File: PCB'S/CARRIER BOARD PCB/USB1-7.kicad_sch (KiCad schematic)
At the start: 7 parts, among them J10 USB_A - 4, J11 USB_A - 5, J12 USB_A - 6 (For Display), J13 USB_A - 7 (For RTL SDR), J14 USB_A - 2 (Extra/For phone ), J7 USB_A - 1, J9 USB_A - 3

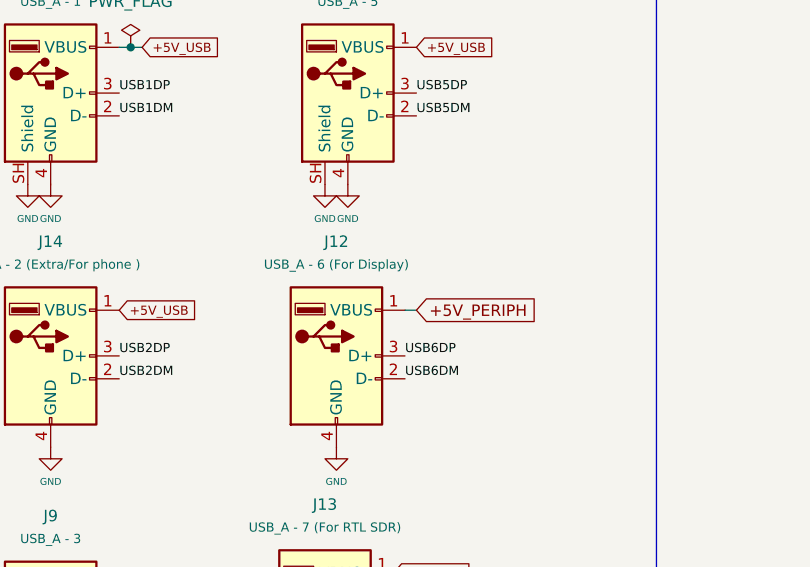
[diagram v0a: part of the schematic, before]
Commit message: ain
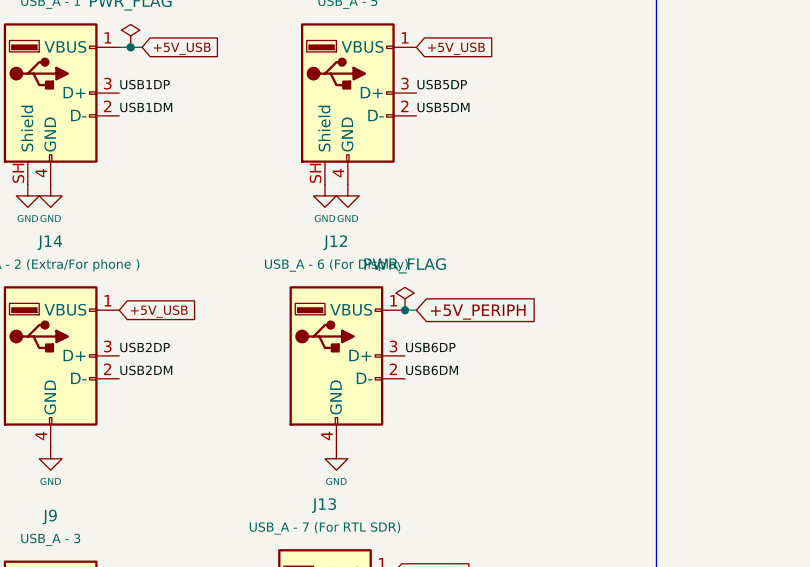
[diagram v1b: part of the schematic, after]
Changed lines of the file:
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@@
+		(color 0 0 0 0)
+	)
+	(junction
+		(at 78.74 92.71)
+		(diameter 0)
 		(color 0 0 0 0)
 	)
@@
 					(unit 1)
 				)
+			)
+		)
+	)
+	(symbol
+		(lib_id "power:PWR_FLAG")
+		(at 78.74 92.71 0)
+		(unit 1)
+		(body_style 1)
+		(exclude_from_sim no)
+		(in_bom yes)
+		(on_board yes)
+		(in_pos_files yes)
+		(dnp no)
+		(fields_autoplaced yes)
+		(property "Reference" "#FLG04"
+			(at 78.74 90.805 0)
+			(hide yes)
+			(show_name no)
+			(do_not_autoplace no)
+			(effects
+				(font
+					(size 1.27 1.27)
+				)
+			)
+		)
+		(property "Value" "PWR_FLAG"
+			(at 78.74 87.63 0)
+			(show_name no)
+			(do_not_autoplace no)
+			(effects
+				(font
+					(size 1.27 1.27)
+				)
+			)
+		)
+		(property "Footprint" "Package_SO:TSSOP-28_4.4x9.7mm_P0.65mm"
+			(at 78.74 92.71 0)
+			(hide yes)
+			(show_name no)
+			(do_not_autoplace no)
+			(effects
+				(font
+					(size 1.27 1.27)
+				)
+			)
+		)
+		(property "Datasheet" ""
+			(at 78.74 92.71 0)
+			(hide yes)
+			(show_name no)
+			(do_not_autoplace no)
+			(effects
+				(font
+					(size 1.27 1.27)
+				)
+			)
+		)
+		(property "Description" "Special symbol for telling ERC where power comes from"
+			(at 78.74 92.71 0)
+			(hide yes)
+			(show_name no)
+			(do_not_autoplace no)
+			(effects
+				(font
+					(size 1.27 1.27)
+				)
+			)
+		)
+		(pin "1"
+		)
+		(instances
+			(project "carrier-orange pi zero 3w"
+				(path "/eed97ac6-b1d8-4052-bc40-1c993c6f2bcf/dc032c8e-044c-497e-baa0-c9bab8568430/be3c0006-2c92-4f50-94ad-ec8e1904ad37"
+					(reference "#FLG04")
+					(unit 1)
+				)
